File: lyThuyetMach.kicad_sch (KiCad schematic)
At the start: 34 parts, among them J1 USB_C_Receptacle_PowerOnly_6P, J2 Voltage_Booster, J4 Out_LED, Q1 BC547, Q2 BC547, Q3 BC547, Q4 BC547, Q5 BC547, Q6 BC547, Q7 TIP122, SW1 SW_SPDT, SW2 SW_SPDT

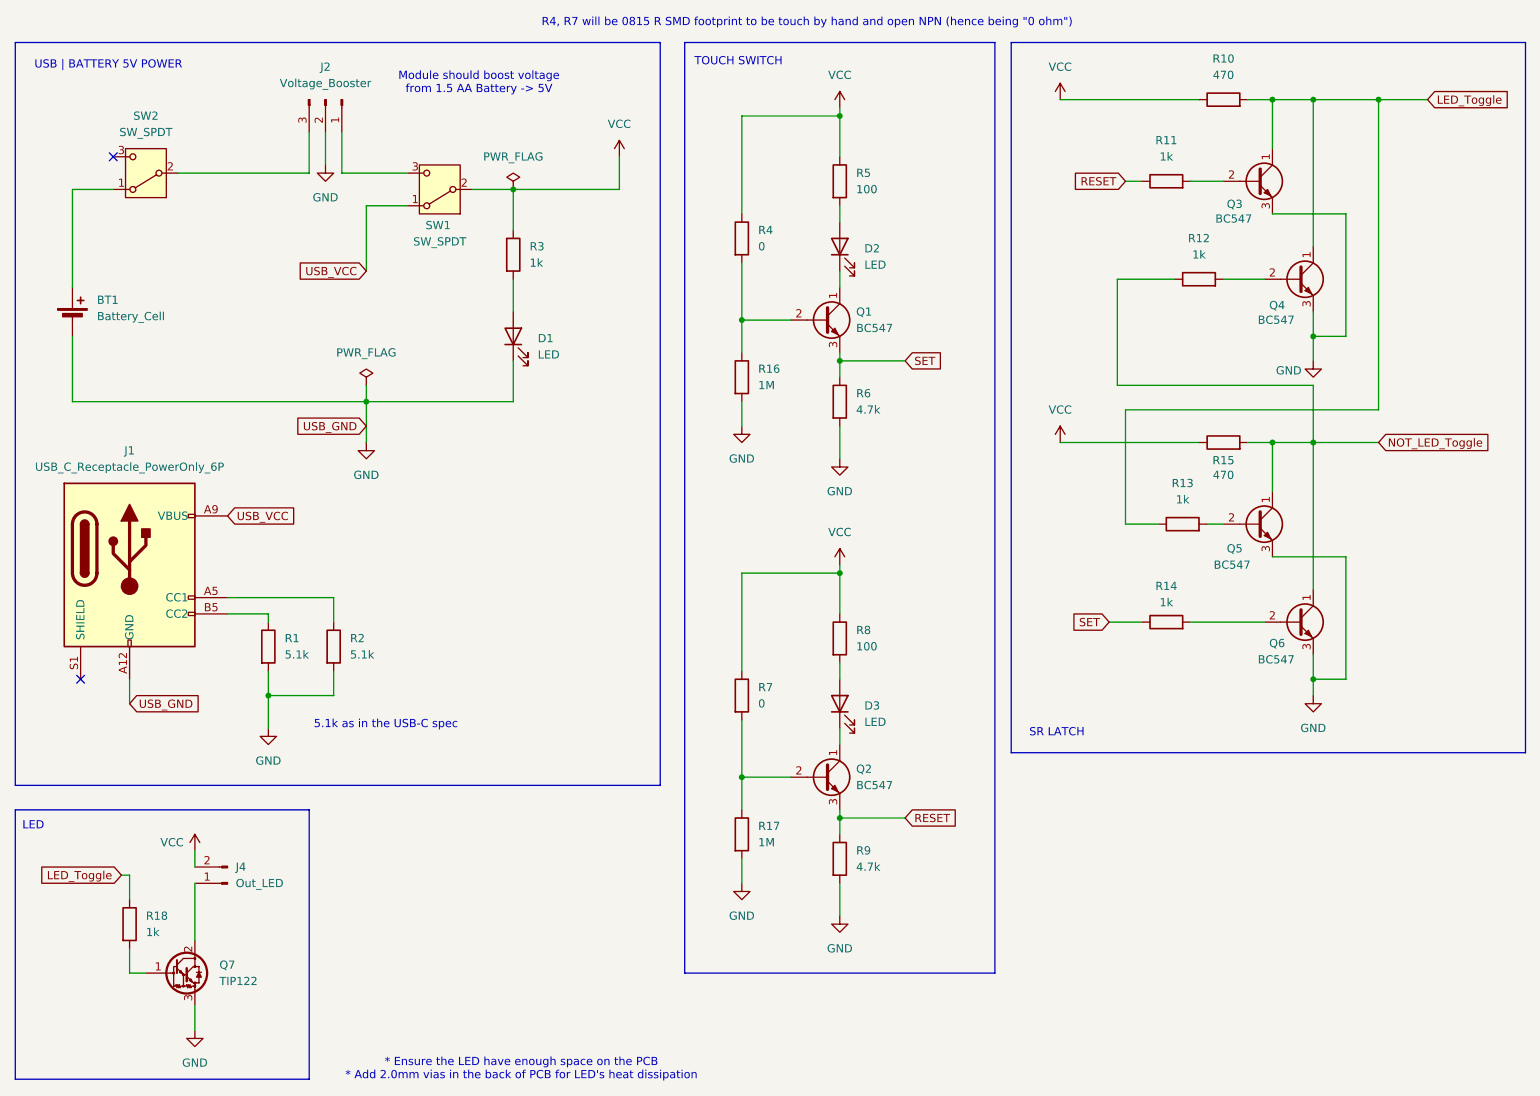
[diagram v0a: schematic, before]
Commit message: Add files via upload
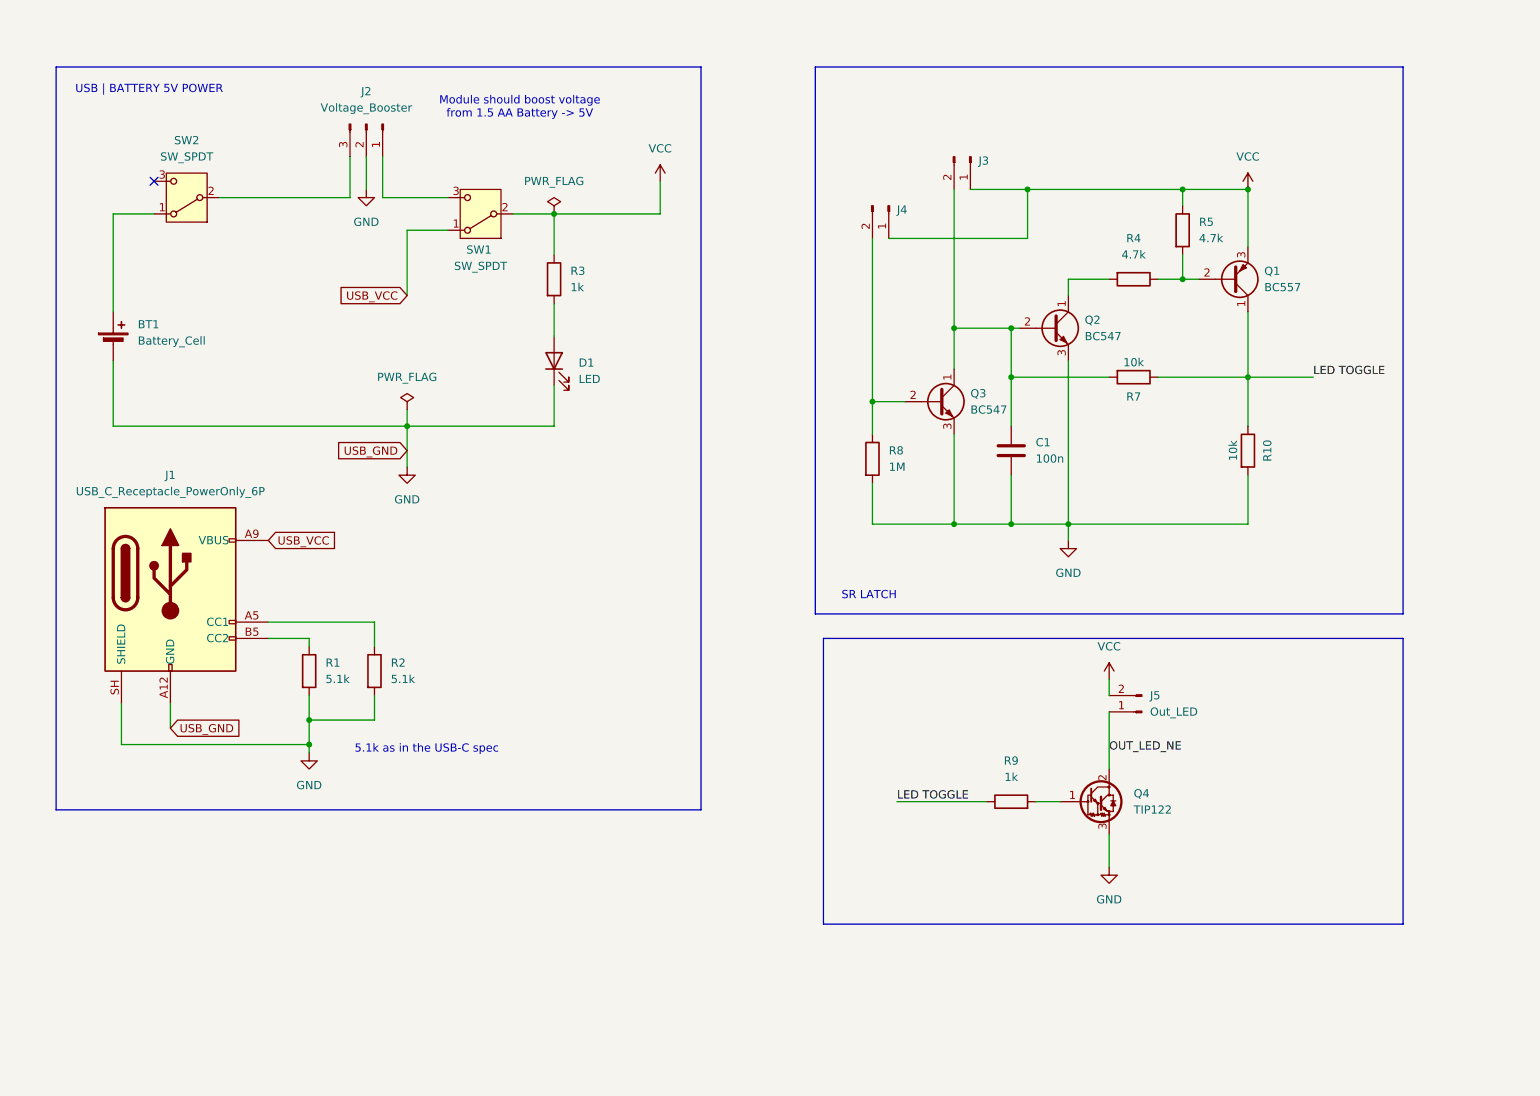
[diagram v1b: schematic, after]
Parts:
- removed D2, D3: LED, LED_THT:LED_D5.0mm_FlatTop, symbol Device:LED
- removed Q1, Q4, Q5, Q6: BC547, Package_TO_SOT_THT:TO-92_Inline, symbol Transistor_BJT:BC547
- removed Q7: TIP122, Package_TO_SOT_THT:TO-220-3_Vertical, symbol Transistor_BJT:TIP122
- removed R11, R12, R13, R14, R18: 1k, Resistor_THT:R_Axial_DIN0207_L6.3mm_D2.5mm_P10.16mm_Horizontal, symbol Device:R
- removed R15: 470, Resistor_THT:R_Axial_DIN0207_L6.3mm_D2.5mm_P10.16mm_Horizontal, symbol Device:R
- removed R16, R17: 1M, Resistor_THT:R_Axial_DIN0207_L6.3mm_D2.5mm_P10.16mm_Horizontal, symbol Device:R
- removed R6: 4.7k, Resistor_THT:R_Axial_DIN0207_L6.3mm_D2.5mm_P10.16mm_Horizontal, symbol Device:R
- added C1: 100n, Capacitor_THT:C_Radial_D5.0mm_H5.0mm_P2.00mm, symbol Device:C
- added J3: Conn_01x02_Pin, Resistor_SMD:R_0815_2038Metric_Pad1.20x4.05mm_HandSolder, symbol Connector:Conn_01x02_Pin
- added J5: Out_LED, Connector_PinHeader_2.54mm:PinHeader_1x02_P2.54mm_Vertical, symbol Connector:Conn_01x02_Pin
- added Q1: BC557, Package_TO_SOT_THT:TO-92_Inline, symbol Transistor_BJT:BC557
- added Q4: TIP122, Package_TO_SOT_THT:TO-220-3_Vertical, symbol Transistor_BJT:TIP122
- J4: value Out_LED -> Conn_01x02_Pin; footprint Connector_PinHeader_2.54mm:PinHeader_1x02_P2.54mm_Vertical -> Resistor_SMD:R_0815_2038Metric_Pad1.20x4.05mm_HandSolder
- R10: value 470 -> 10k
- R4: value 0 -> 4.7k; footprint Resistor_SMD:R_0815_2038Metric_Pad1.20x4.05mm_HandSolder -> Resistor_THT:R_Axial_DIN0207_L6.3mm_D2.5mm_P10.16mm_Horizontal
- R5: value 100 -> 4.7k
- R7: value 0 -> 10k; footprint Resistor_SMD:R_0815_2038Metric_Pad1.20x4.05mm_HandSolder -> Resistor_THT:R_Axial_DIN0207_L6.3mm_D2.5mm_P10.16mm_Horizontal
- R8: value 100 -> 1M
- R9: value 4.7k -> 1k
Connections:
- net GND: now also J1.SH (SHIELD), Q2.3 (E), R10.2, R8.2, C1.2, Q4.3 (E); no longer R9.2
- net VCC: now also J4.1 (Pin_1), J3.1 (Pin_1), J5.2 (Pin_2), Q1.3 (E); no longer J4.2 (Pin_2), R10.1, R4.1, R7.1, R8.1
- net at R4.2: now also Q2.1 (C)
- net at R5.2: now also R4.1, Q1.2 (B)
- net at Q3.2 (B): now also J4.2 (Pin_2), R8.1
- net at Q2.2 (B), R7.2: now also Q3.1 (C), C1.1, J3.2 (Pin_2)
- removed net LED_Toggle: Q3.1 (C), R10.2
- net RESET renamed LED TOGGLE
- net LED TOGGLE: now also R10.1, R7.1, Q1.1 (C); no longer Q2.3 (E)
- new net: Q4.1 (B), R9.2
- new net OUT_LED_NE: J5.1 (Pin_1), Q4.2 (C)
- no-connect marks 2 -> 1
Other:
- note removed: "* Ensure the LED have enough space on the PCB * Add 2.0mm vias in the back of PCB for LED's heat dissipation"
- note removed: "LED"
- note removed: "R4, R7 will be 0815 R SMD footprint to be touch by hand and open NPN (hence being "0 ohm")"
- note removed: "TOUCH SWITCH"
- moved on the sheet: BT1, D1, J1, J2, R1, R2, R3, SW1, SW2
